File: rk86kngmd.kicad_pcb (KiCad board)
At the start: 2 copper layers, 226.2 x 62.5 mm, 39 parts, among them P1 GND, P10 TR00, P11 WPRT, P12 RD_DATA, P13 SIDE, P14 READY, P2 +5V, P3 IP, P4 DISC_A, P5 DISC_B, P6 DIR, P7 STEP, P8 WR_DATA, P9 WR_GATE, X1 ОНп-КС-23

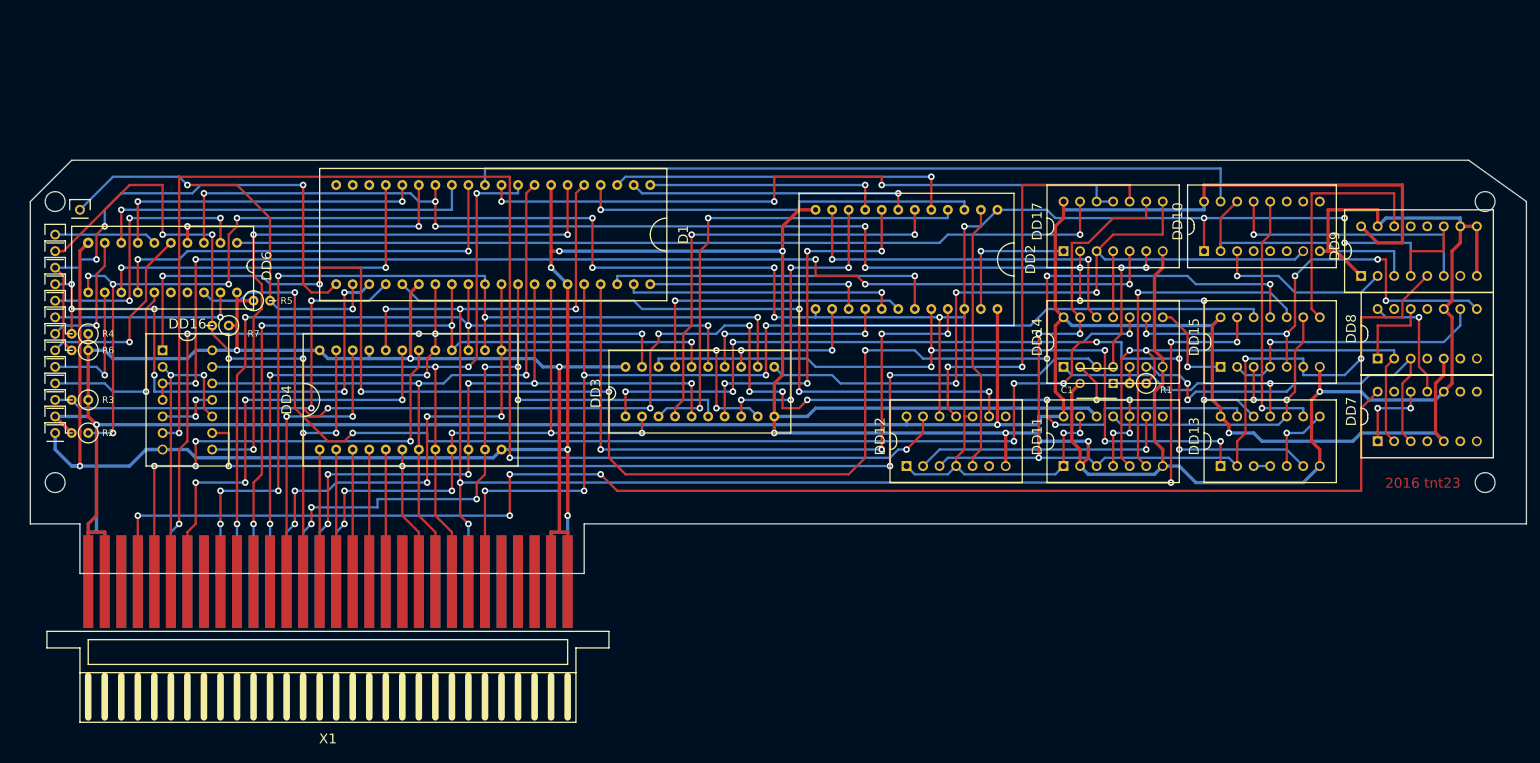
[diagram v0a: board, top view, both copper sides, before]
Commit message: .
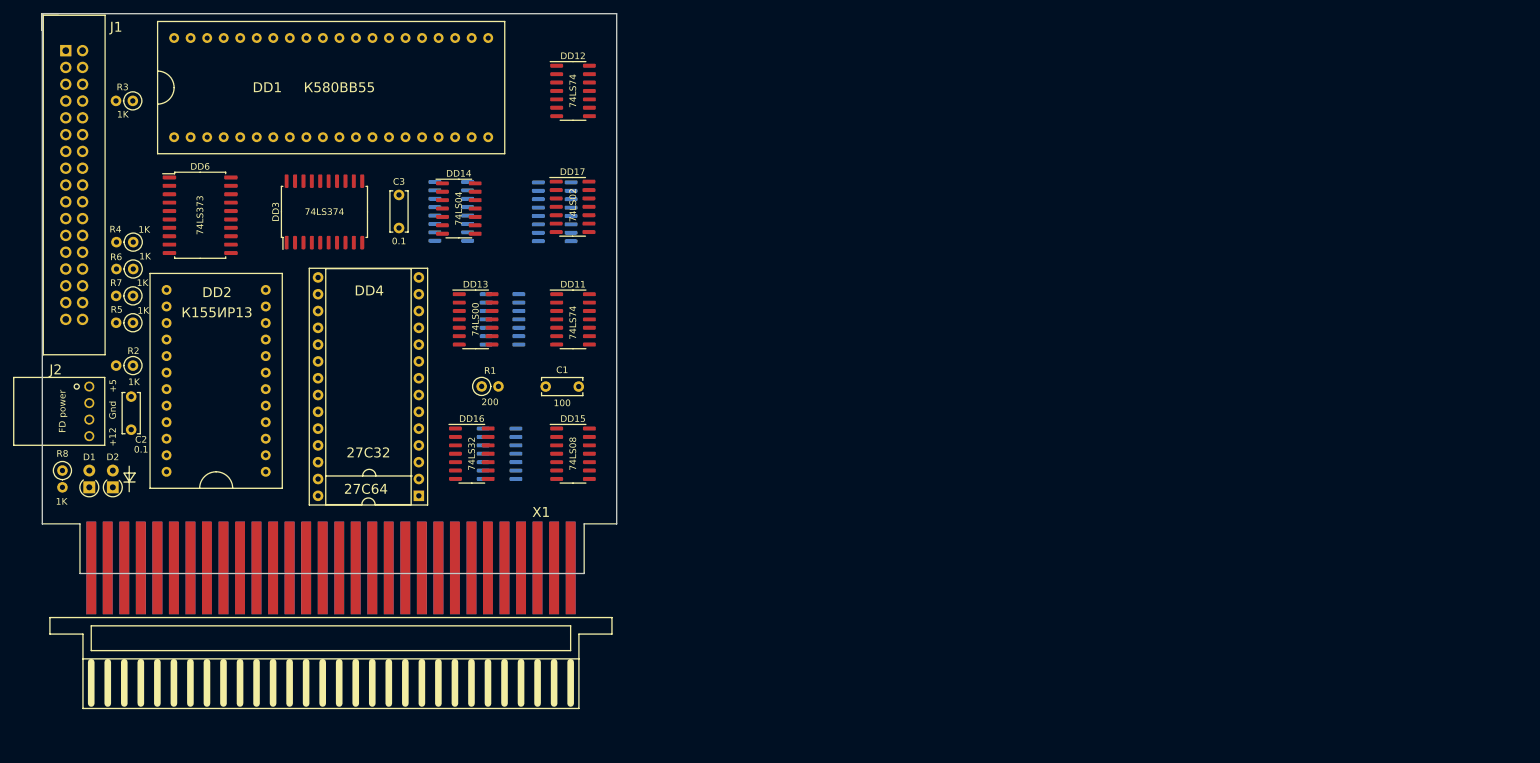
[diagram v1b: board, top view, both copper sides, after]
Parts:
- removed P1: GND, Pin_Headers:Pin_Header_Straight_1x01
- removed P10: TR00, Pin_Headers:Pin_Header_Straight_1x01
- removed P11: WPRT, Pin_Headers:Pin_Header_Straight_1x01
- removed P12: RD_DATA, Pin_Headers:Pin_Header_Straight_1x01
- removed P13: SIDE, Pin_Headers:Pin_Header_Straight_1x01
- removed P14: READY, Pin_Headers:Pin_Header_Straight_1x01
- removed P2: +5V, Pin_Headers:Pin_Header_Straight_1x01
- removed P3: IP, Pin_Headers:Pin_Header_Straight_1x01
- removed P4: DISC_A, Pin_Headers:Pin_Header_Straight_1x01
- removed P5: DISC_B, Pin_Headers:Pin_Header_Straight_1x01
- removed P6: DIR, Pin_Headers:Pin_Header_Straight_1x01
- removed P7: STEP, Pin_Headers:Pin_Header_Straight_1x01
- removed P8: WR_DATA, Pin_Headers:Pin_Header_Straight_1x01
- removed P9: WR_GATE, Pin_Headers:Pin_Header_Straight_1x01
- added C2: 0.1, Capacitor_THT:C_Disc_D6.0mm_W2.5mm_P5.00mm, F.Cu at (56.2, 106.2)
- added C3: 0.1, Capacitor_THT:C_Disc_D6.0mm_W2.5mm_P5.00mm, F.Cu at (96.8, 80.8)
- added D2: 2N4148, Diode_THT:D_A-405_P2.54mm_Vertical_AnodeUp, F.Cu at (53.5, 120.0)
- added DD1: К580ВВ55, rk86kngmd:DIP40-2.5mm, F.Cu at (86.5, 59.5)
- added J1: Conn_02x17_Odd_Even, Connector_IDC:IDC-Header_2x17_P2.54mm_Vertical, F.Cu at (46.4, 53.9)
- added J2: FD power, rk86kngmd:171826-4, F.Cu at (49.9, 104.7)
- added R8: 1K, Resistor_THT:R_Axial_DIN0207_L6.3mm_D2.5mm_P2.54mm_Vertical, F.Cu at (45.9, 117.4)
- C1: footprint Capacitors_ThroughHole:C_Disc_D6_P5 -> Capacitor_THT:C_Disc_D6.0mm_W2.5mm_P5.00mm
- D1: value К580ВВ55 -> 2N4148; footprint rk86kngmd:DIP40-2.5mm -> Diode_THT:D_A-405_P2.54mm_Vertical_AnodeUp
- DD10: value К555ИД4 -> 74LS155; footprint DIP16-2.5mm -> Package_SO:SOIC-16_3.9x9.9mm_P1.27mm; moved to B.Cu
- DD11, DD12: value К555ТМ2 -> 74LS74; footprint rk86ngmd:DIP14-2.5mm -> Package_SO:SOIC-14_3.9x8.7mm_P1.27mm
- DD13: value К555ЛА3 -> 74LS00; footprint rk86ngmd:DIP14-2.5mm -> Package_SO:SOIC-14_3.9x8.7mm_P1.27mm
- DD14: value К555ЛН1 -> 74LS04; footprint rk86ngmd:DIP14-2.5mm -> Package_SO:SOIC-14_3.9x8.7mm_P1.27mm
- DD15: value К555ЛИ1 -> 74LS08; footprint rk86ngmd:DIP14-2.5mm -> Package_SO:SOIC-14_3.9x8.7mm_P1.27mm
- DD16: value К555ЛЛ1 -> 74LS32; footprint rk86ngmd:DIP14-2.5mm -> Package_SO:SOIC-14_3.9x8.7mm_P1.27mm
- DD17: value К555ЛЕ1 -> 74LS02; footprint DIP14-2.5mm -> Package_SO:SOIC-14_3.9x8.7mm_P1.27mm
- DD2: value К555ИР13 -> К155ИР13; footprint DIP24-2.5mm -> rk86kngmd:DIP24-2.5mm
- DD3: value К555ИР23 -> 74LS374; footprint DIP20-2.5mm -> Package_SO:SOIC-20W_7.5x12.8mm_P1.27mm
- DD4: value 2716 -> 27C64; footprint rk86ngmd:DIP24-2.5mm -> Package_DIP:DIP-28_W15.24mm_Socket
- DD6: value К555ИР22 -> 74LS373; footprint rk86ngmd:DIP20-2.5mm -> Package_SO:SOIC-20W_7.5x12.8mm_P1.27mm
- DD7, DD8: value К555ИЕ5 -> 74LS93; footprint rk86ngmd:DIP14-2.5mm -> Package_SO:SOIC-14_3.9x8.7mm_P1.27mm; moved to B.Cu
- DD9: value К555ИЕ7 -> 74LS193; footprint rk86ngmd:DIP16-2.5mm -> Package_SO:SOIC-16_3.9x9.9mm_P1.27mm; moved to B.Cu
- R1, R2, R3, R4, R5, R7: footprint rk86ngmd:Resistor_Vertical_RM2_5mm -> Resistor_THT:R_Axial_DIN0207_L6.3mm_D2.5mm_P2.54mm_Vertical
- R6: footprint Resistor_Vertical_RM2_5mm -> Resistor_THT:R_Axial_DIN0207_L6.3mm_D2.5mm_P2.54mm_Vertical
- X1: footprint rk86ngmd:ОНп-КС-23 -> rk86kngmd:ОНп-КС-23
- moved DD7 153.7 mm to (112.0, 114.9), turned to 0 degrees
- moved DD8 152.6 mm to (112.4, 94.6), turned to 0 degrees
- moved DD13 132.9 mm to (108.3, 94.6), turned to 0 degrees
- moved DD9 122.3 mm to (120.3, 78.3), turned to 0 degrees
- moved DD15 121.2 mm to (123.1, 114.9), turned to 0 degrees
- moved DD10 114.0 mm to (104.7, 78.2), turned to 0 degrees
- moved DD14 111.8 mm to (105.8, 77.8), turned to 0 degrees
- moved DD2 105.8 mm to (61.6, 97.6), turned to 180 degrees
- moved R1 98.0 mm to (109.2, 104.7), turned to 0 degrees
- moved DD17 94.6 mm to (123.0, 77.6), turned to 0 degrees
- moved DD11 94.5 mm to (123.1, 94.6), turned to 0 degrees
- moved C1 85.8 mm to (118.9, 104.7), turned to 0 degrees
- moved DD12 81.9 mm to (123.1, 60.0), turned to 0 degrees
- moved D1 72.1 mm to (49.9, 120.0), turned to 90 degrees
- moved DD3 58.0 mm to (85.5, 78.3)
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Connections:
- D1 pad 1: Net-(D1-Pad1) -> /CS1
- D1 pad 2: Net-(D1-Pad2) -> /CS12
- DD16 pad 8: Net-(D1-Pad6) -> Net-(DD1-Pad6)
- DD2 pad 15: Net-(D1-Pad40) -> Net-(DD1-Pad40)
- DD2 pad 17: Net-(D1-Pad39) -> Net-(DD1-Pad39)
- DD2 pad 19: Net-(D1-Pad38) -> Net-(DD1-Pad38)
- DD2 pad 21: Net-(D1-Pad37) -> Net-(DD1-Pad37)
- DD2 pad 3: Net-(D1-Pad4) -> Net-(DD1-Pad4)
- DD2 pad 5: Net-(D1-Pad3) -> Net-(DD1-Pad3)
- DD2 pad 7: Net-(D1-Pad2) -> Net-(DD1-Pad2)
- DD2 pad 9: Net-(D1-Pad1) -> Net-(DD1-Pad1)
- DD4 pad 1: /A7 -> +5V
- DD4 pad 10: /D1 -> /A0
- DD4 pad 11: /D2 -> /D0
- DD4 pad 12: GND -> /D1
- DD4 pad 13: /D3 -> /D2
- DD4 pad 14: /D4 -> GND
- DD4 pad 15: /D5 -> /D3
- DD4 pad 16: /D6 -> /D4
- DD4 pad 17: /D7 -> /D5
- DD4 pad 18: /CS1 -> /D6
- DD4 pad 19: /A10 -> /D7
- DD4 pad 2: /A6 -> GND
- DD4 pad 20: /RD -> /CS12
- DD4 pad 21: +5V -> /A10
- DD4 pad 22: /A9 -> /RD
- DD4 pad 23: /A8 -> /A11
- DD4 pad 24: +5V -> /A9
- DD4 pad 3: /A5 -> /A7
- DD4 pad 4: /A4 -> /A6
- DD4 pad 5: /A3 -> /A5
- DD4 pad 6: /A2 -> /A4
- DD4 pad 7: /A1 -> /A3
- DD4 pad 8: /A0 -> /A2
- DD4 pad 9: /D0 -> /A1
- X1 pad B11: Net-(X1-PadB11) -> +12V
- X1 pad B23: Net-(X1-PadB23) -> /A11
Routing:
- net GND: track 608.9 -> 0.00 mm, vias 10 -> 0
- net +5V: track 574.7 -> 0.00 mm, vias 6 -> 0
- net Net-(DD10-Pad1): track 372.7 -> 0.00 mm, vias 16 -> 0
- net Net-(DD15-Pad11): track 247.4 -> 0.00 mm, vias 8 -> 0
- net RD_DATA: track 247.0 -> 0.00 mm, vias 13 -> 0
- net /RD: track 238.5 -> 0.00 mm, vias 8 -> 0
- net /WRDATA: track 219.4 -> 0.00 mm, vias 8 -> 0
- net /OSC: track 218.3 -> 0.00 mm, vias 4 -> 0
- net /WRGATE: track 202.8 -> 0.00 mm, vias 9 -> 0
- net Net-(DD12-Pad13): track 200.3 -> 0.00 mm, vias 3 -> 0
- net Net-(DD16-Pad3): track 175.5 -> 0.00 mm, vias 5 -> 0
- net /A2: track 175.1 -> 0.00 mm, vias 4 -> 0
- net /WR: track 169.8 -> 0.00 mm, vias 5 -> 0
- net Net-(DD11-Pad3): track 159.7 -> 0.00 mm, vias 5 -> 0
- net /D4: track 146.2 -> 0.00 mm, vias 6 -> 0
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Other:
- board size 226.2 x 62.5 mm -> 86.9 x 84.7 mm
- board text added: "+12"
- board text added: "+5"
- board text added: "Gnd"
- board text added: "RK86 FD Controller"
- board text added: "©2020 SDS"
- board text removed: "2016 tnt23"
